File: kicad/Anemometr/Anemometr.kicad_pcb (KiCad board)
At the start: 2 copper layers, 44.9 x 45.2 mm, 163 parts, among them J10 +Z3, J11 -Z3, J12 +Z4, J13 -Z4, J14 SWD, J15 SWC, J18 1 TxD+, J19 2 TxD-, J2 Conn_01x01_Female, J20 3 RxD+, J21 4-5, J23 6 RxD-, J24 7-8, J3 RST, J36 TMP117, J37 TMP117, J38 TMP117, J39 TMP117, J4 TxD, J5 RxD, J6 +Z1, J7 -Z1, J8 +Z2, J9 -Z2, Q1 5N10, U1 TS5A3166DBVR, U10 LM2734Y, U2 LMV7239, U3 TS5A3166DBVR, U4 TS5A3166DBVR, U5 STM32F103C8Tx, U6 TS5A3166DBVR, U7 LM2734Y, U8 MCP1700-5002E, Y1 8MHz, Y2 25MHz

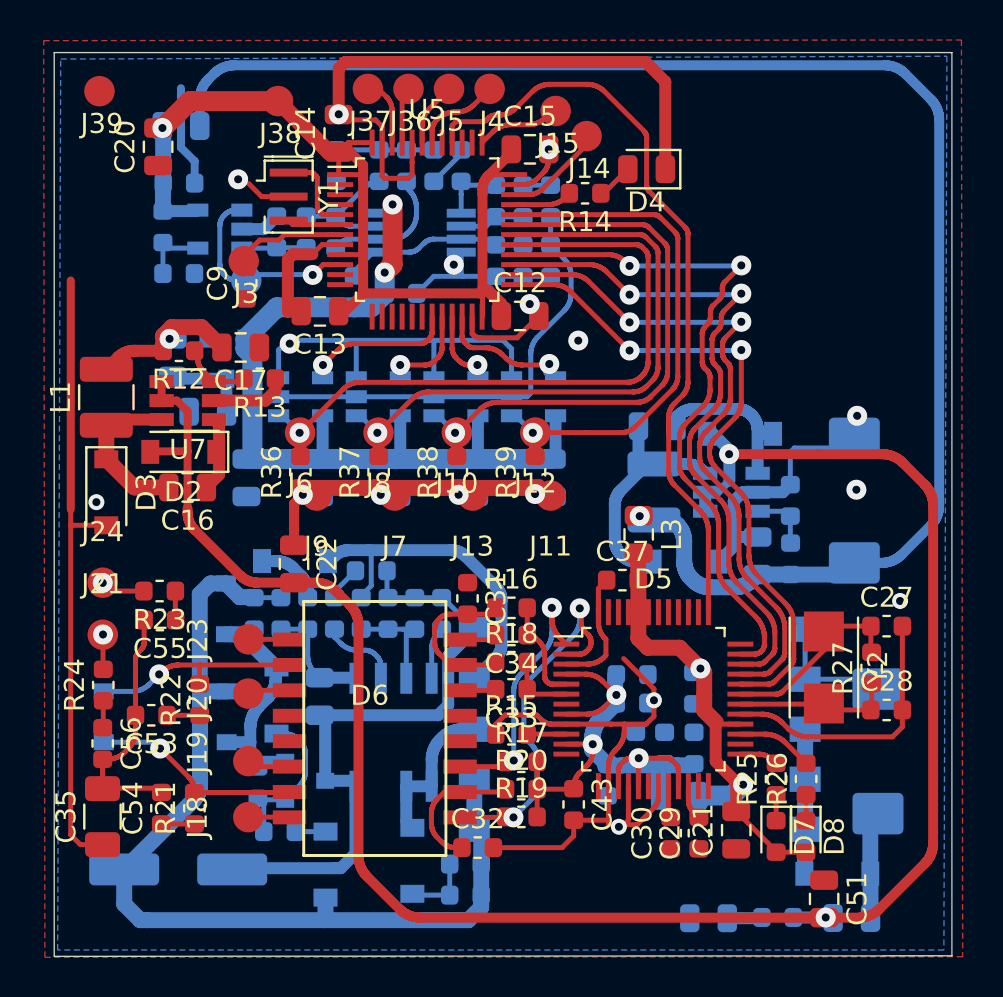
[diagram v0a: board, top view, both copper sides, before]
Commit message: изменено:      kicad/Anemometr/Anemometr.kicad_pcb 	изменено:      kicad/Anemometr/Anemometr.kicad_pcb-bak 	изменено:      kicad/Anemometr/Anemometr.sch 	изменено:      kicad/Anemometr/Anemometr.sch-bak 	изменено:      stm32cubeide/Anemometer/Core/Inc/main.h 	изменено:      stm32cubeide/Anemometer/Core/Inc/wizchip_conf.h 	изменено:      stm32cubeide/Anemometer/Core/Src/dhcp.c 	изменено:      stm32cubeide/Anemometer/Core/Src/main.c 	изменено:      stm32cubeide/Anemometer/Release/Anemometer.bin 	изменено:      stm32cubeide/Anemometer/Release/Anemometer.elf 	изменено:      stm32cubeide/Anemometer/Release/Anemometer.list 	изменено:      stm32cubeide/Anemometer/Release/Anemometer.map 	изменено:      stm32cubeide/Anemometer/Release/Core/Src/main.o 	изменено:      stm32cubeide/Anemometer/Release/Core/Src/main.su 	изменено:      stm32cubeide/Anemometer/Release/Core/Src/stm32f1xx_it.o
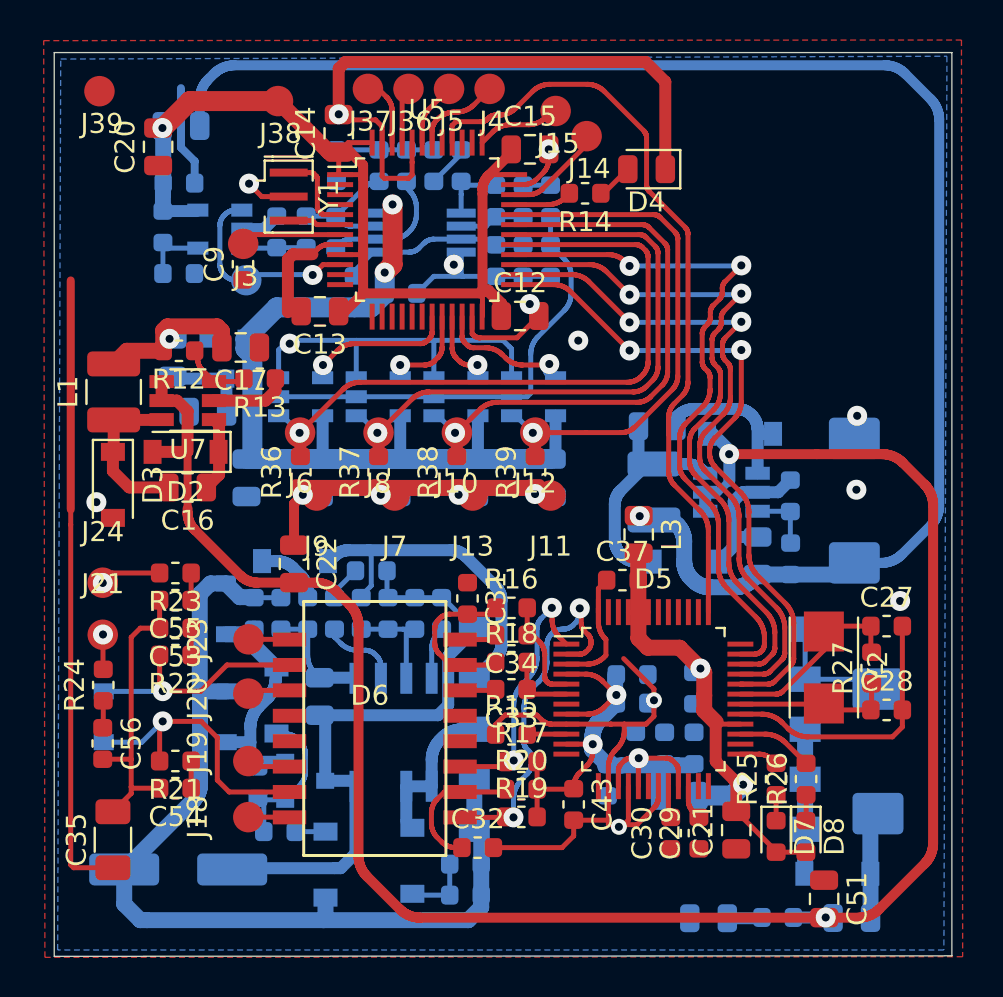
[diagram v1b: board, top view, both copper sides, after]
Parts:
- moved C53 4.52 mm to (24.9, 88.4)
- moved R21 2.55 mm to (24.9, 95.0), turned to 180 degrees
- moved R22 2.55 mm to (24.9, 89.7), turned to 180 degrees
- moved C35 1.27 mm to (21.8, 99.0)
- moved C55 1.26 mm to (24.9, 87.0)
- moved C54 1.22 mm to (24.9, 96.4), turned to 180 degrees
- moved R23 1.20 mm to (24.9, 85.6)
- moved C9 0.97 mm to (28.3, 70.2)
- moved J3 0.86 mm to (28.3, 69.2)
- moved D3 0.49 mm to (21.8, 81.2)
- moved L1 0.45 mm to (21.8, 76.6)
- moved R44 0.23 mm to (55.7, 81.8)
- moved D2 0.11 mm to (25.4, 79.6)
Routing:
- net GND: track 200.1 -> 195.2 mm
- net Net-(D6-Pad15): track 10.6 -> 14.5 mm
- net Net-(C35-Pad2): track 12.6 -> 15.0 mm
- net Net-(D6-Pad10): track 10.7 -> 11.7 mm
- net Net-(D10-Pad2): track 2.23 -> 3.04 mm

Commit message: изменено:      kicad/Anemometr/Anemometr-cache.lib 	изменено:      kicad/Anemometr/Anemometr.kicad_pcb 	изменено:      kicad/Anemometr/Anemometr.kicad_pcb-bak 	изменено:      kicad/Anemometr/Anemometr.sch 	изменено:      kicad/Anemometr/Anemometr.sch-bak
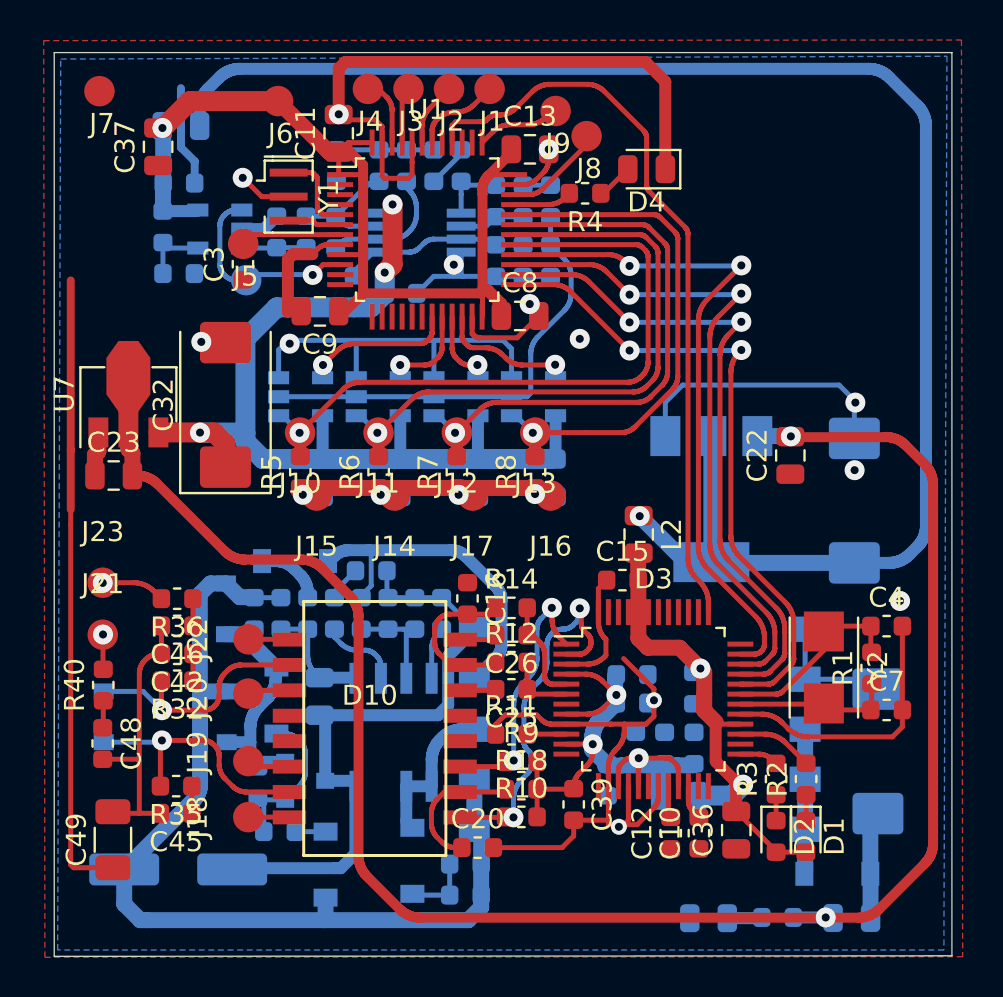
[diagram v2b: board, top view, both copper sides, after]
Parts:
- removed the C16 at (25.5, 81.3)
- removed the C17 at (28.2, 74.3)
- removed the C19 at (28.5, 80.9)
- removed the C50 at (49.0, 78.3)
- removed the C51 at (57.4, 101.9)
- removed C57: 22uF, Capacitor_SMD:C_0805_2012Metric
- removed D19, D20: MBR0540, Diode_SMD:D_SOD-123
- removed the D2 at (25.4, 79.6)
- removed the D3 at (21.8, 81.2)
- removed the L1 at (21.8, 76.6)
- removed the L2 at (24.8, 74.9)
- removed L6: 22uH, Inductor_SMD:L_1210_3225Metric
- removed the R12 at (25.1, 74.5)
- removed the R13 at (29.1, 75.9)
- removed the R35 at (55.7, 84.9)
- removed R44: 10k, Resistor_SMD:R_0603_1608Metric
- removed U10: LM2734Y, Package_TO_SOT_SMD:TSOT-23-6
- removed the U8 at (27.5, 74.9)
- added C32: 1000uF, Capacitor_Tantalum_SMD:CP_EIA-7343-15_Kemet-W, F.Cu at (27.4, 77.2)
- added U6: NCP1117-3.3, Package_TO_SOT_SMD:SOT-223-3_TabPin2, B.Cu at (51.7, 81.9)
- C23: renamed from C18; moved to F.Cu
- L4: renamed from L5; value 47uH -> 10uH
- U7: value LM2734Y -> MCP1703A-5002; footprint Package_TO_SOT_SMD:TSOT-23-6 -> Package_TO_SOT_SMD:SOT-89-3
- moved C22 25.4 mm to (55.7, 79.7), turned to 90 degrees
- moved C23 5.69 mm to (21.8, 80.7)
- moved U7 2.97 mm to (22.6, 77.1), turned to 90 degrees
- moved C42 1.29 mm to (25.0, 89.7)
- moved C46 1.29 mm to (25.0, 88.3)
- moved R32 1.29 mm to (25.0, 91.0)
- moved R36 1.29 mm to (25.0, 86.9)
- moved C45 1.26 mm to (25.0, 97.6)
- moved R35 1.26 mm to (25.0, 96.3)
- renumbered C23 to C1, C29 to C10, C14 to C11, C30 to C12, C15 to C13, C36 to C14, C37 to C15, C31 to C16, C1 to C17, C4 to C18, C45 to C19, C24 to C2, C32 to C20, C8 to C21, C46 to C24, C33 to C25, C34 to C26, C38 to C27, C39 to C28, C52 to C29, C9 to C3, C58 to C30, C40 to C31, C47 to C33, C6 to C34, C41 to C35, C21 to C36, C20 to C37, C42 to C38, C43 to C39, C27 to C4, C3 to C40, C7 to C41, C53 to C42, C44 to C43, C48 to C44, C54 to C45, C55 to C46, C5 to C47, C56 to C48, C35 to C49, C25 to C5, C49 to C50, C2 to C51, C26 to C6, C28 to C7, C12 to C8, C13 to C9, D8 to D1, D6 to D10, D12 to D11, D9 to D12, D15 to D14, D10 to D15, D14 to D16, D7 to D2, D5 to D3, D18 to D5, D16 to D6, D1 to D7, D11 to D8, D17 to D9, J4 to J1, J6 to J10, J8 to J11, J10 to J12, J12 to J13, J7 to J14, J9 to J15, J11 to J16, J13 to J17, J5 to J2, J23 to J22, J24 to J23, J2 to J24, J36 to J3, J37 to J4, J3 to J5, J38 to J6, J39 to J7, J14 to J8, J15 to J9, L4 to L1, L3 to L2, L7 to L3, R27 to R1, R19 to R10, R15 to R11, R18 to R12, R7 to R13, R16 to R14, R43 to R15, R1 to R16, R8 to R17, R20 to R18, R28 to R19, R26 to R2, R5 to R20, R29 to R21, R30 to R22, R40 to R23, R42 to R24, R4 to R25, R31 to R26, R32 to R27, R33 to R28, R6 to R29, R25 to R3, R41 to R30, R9 to R31, R22 to R32, R2 to R33, R21 to R35, R23 to R36, R10 to R37, R3 to R38, R11 to R39, R14 to R4, R24 to R40, R36 to R5, R37 to R6, R38 to R7, R39 to R8, R17 to R9, U5 to U1, U1 to U2, U6 to U5, U2 to U8
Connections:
- C23 pad 2: Net-(C18-Pad2) (its old number) -> Net-(C22-Pad2)
- U7 pad 1: Net-(C16-Pad1) -> GND
- U7 pad 2: GND -> Net-(C22-Pad2)
- U7 pad 3: Net-(R12-Pad1) -> +5VA
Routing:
- net Net-(C50-Pad2): track 11.3 -> 0.00 mm
- net Net-(C50-Pad1) (its old number): track 8.20 -> 0.00 mm
- net Net-(C16-Pad2) (its old number): track 8.12 -> 0.00 mm
- net Net-(C17-Pad2): track 8.10 -> 0.00 mm, vias 1 -> 0
- net +5VA: track 44.5 -> 50.4 mm, vias 2 -> 3
- net Net-(C22-Pad2): track 99.9 -> 95.0 mm
- net Net-(C18-Pad2) (its old number): track 4.40 -> 0.00 mm
- net Net-(C30-Pad1): track 78.4 -> 82.2 mm
- net Net-(C16-Pad1): track 3.76 -> 0.00 mm
- net Net-(R12-Pad1): track 3.40 -> 0.00 mm
- net Net-(R35-Pad1): track 3.22 -> 0.00 mm
- net GND: track 195.2 -> 196.8 mm
- net Net-(D10-Pad15): track 14.5 -> 13.3 mm
- net Net-(D3-Pad34): track 34.6 -> 33.7 mm
- net Net-(D3-Pad33): track 34.2 -> 33.3 mm
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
